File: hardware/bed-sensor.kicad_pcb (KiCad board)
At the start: 2 copper layers, 21.3 x 43.2 mm, 46 parts, among them J1 USB_B_Mini, J2 Conn_ARM_JTAG_SWD_10, J3 DM3AT-SF-PEJM5, J4 Conn_01x02, Q1 Q_PMOS_GSD, SW1 SW_Push, U1 MCP73831-2-OT, U2 TLV70218_SOT23-5, U3 AP2112K-3.3, U4 MDBT50Q-1M, U5 PCA9306, U6 ICM-20948, U7 BMP280, Y1 32.768

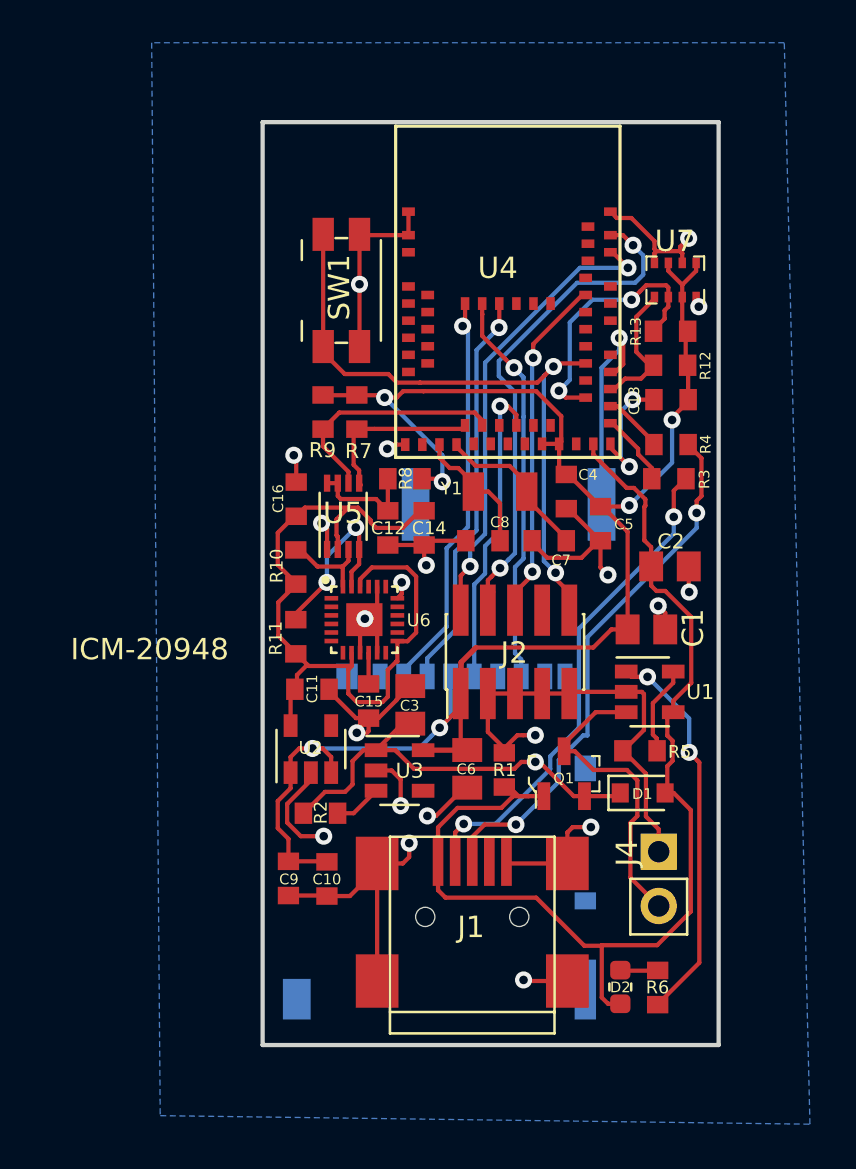
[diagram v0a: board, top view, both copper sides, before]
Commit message: finalized order list
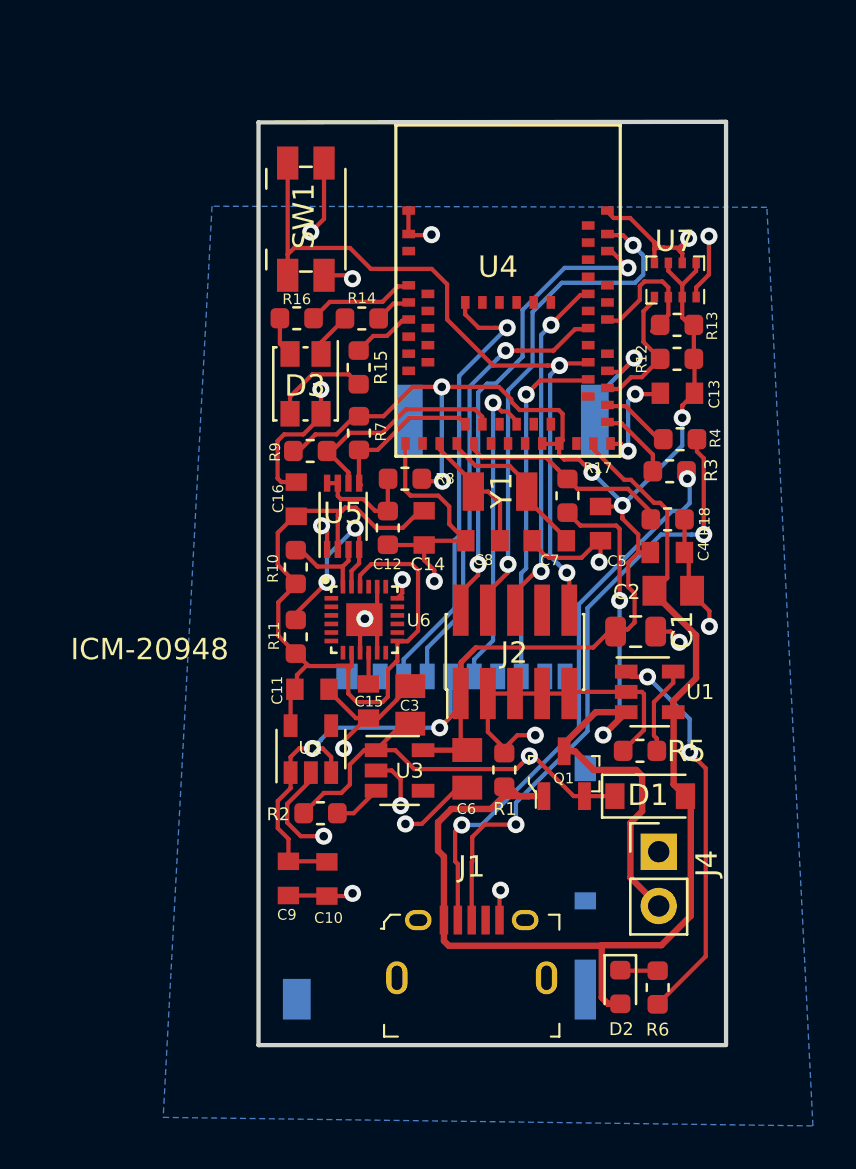
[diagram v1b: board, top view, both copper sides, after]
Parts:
- added D3: LED_RCGB, LED_SMD:LED_Kingbright_AAA3528ESGCT, F.Cu at (138.6, 98.6)
- added R14: 330, Resistor_SMD:R_0603_1608Metric, F.Cu at (141.2, 95.5)
- added R15: 330, Resistor_SMD:R_0603_1608Metric, F.Cu at (141.1, 97.8)
- added R16: 330, Resistor_SMD:R_0603_1608Metric, F.Cu at (138.2, 95.5)
- added R17: 100k, Resistor_SMD:R_0603_1608Metric, F.Cu at (150.8, 103.8)
- added R18: 100k, Resistor_SMD:R_0603_1608Metric, F.Cu at (155.5, 105.0)
- D1: footprint Diodes_SMD:D_0805 -> Diode_SMD:D_SOD-123
- D2: footprint Capacitor_SMD:C_0603_1608Metric -> Diode_SMD:D_0603_1608Metric
- J1: footprint Connectors:USB_Mini-B -> digikey-footprints:USB_Micro_B_Female_10118194-0001LF
- moved C4 5.52 mm to (155.5, 106.5), turned to 0 degrees
- moved BZ1 3.91 mm to (147.8, 100.3)
- moved SW1 3.73 mm to (138.6, 90.9)
- moved R9 1.92 mm to (138.8, 101.8), turned to 180 degrees
- moved C2 1.15 mm to (155.8, 108.3)
- moved R7 0.99 mm to (141.1, 100.9)
- moved C1 0.51 mm to (154.0, 110.2)
- moved R4 0.49 mm to (156.1, 101.2)
- moved R13 0.42 mm to (156.0, 95.8)
- moved R12 0.42 mm to (156.0, 97.4)
- moved C13 0.42 mm to (156.0, 99.0)
- moved D1 0.38 mm to (154.7, 117.9)
- moved R3 0.35 mm to (155.6, 102.7)
- moved J1 0.06 mm to (146.3, 123.7), turned to 0 degrees
- moved U4 0.05 mm to (142.8, 102.0)
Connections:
- J1 pad 4: Net-(J1-Pad4) -> (no net)
- J2 pad 8: Net-(J2-Pad8) -> (no net)
- J3 pad 1: Net-(J3-Pad1) -> (no net)
- J3 pad 8: Net-(J3-Pad8) -> (no net)
- J3 pad SWA: Net-(J3-PadSWA) -> (no net)
- J3 pad SWB: Net-(J3-PadSWB) -> (no net)
- U2 pad 4: Net-(U2-Pad4) -> (no net)
- U3 pad 4: Net-(U3-Pad4) -> (no net)
- U4 pad 10: Net-(U4-Pad10) -> (no net)
- U4 pad 11: Net-(U4-Pad11) -> (no net)
- U4 pad 12: Net-(U4-Pad12) -> (no net)
- U4 pad 13: Net-(U4-Pad13) -> (no net)
- U4 pad 14: Net-(U4-Pad14) -> (no net)
- U4 pad 16: Net-(U4-Pad16) -> (no net)
- U4 pad 20: Net-(U4-Pad20) -> VDIV
- U4 pad 22: Net-(U4-Pad22) -> (no net)
- U4 pad 23: Net-(U4-Pad23) -> (no net)
- U4 pad 24: Net-(U4-Pad24) -> (no net)
- U4 pad 26: Net-(U4-Pad26) -> (no net)
- U4 pad 27: Net-(U4-Pad27) -> (no net)
- U4 pad 29: Net-(U4-Pad29) -> (no net)
- U4 pad 3: Net-(U4-Pad3) -> (no net)
- U4 pad 31: Net-(U4-Pad31) -> (no net)
- U4 pad 36: BMP_SDA -> (no net)
- U4 pad 38: Net-(U4-Pad38) -> SD_MISO
- U4 pad 4: Net-(U4-Pad4) -> B_LED
- U4 pad 41: Net-(U4-Pad41) -> (no net)
- U4 pad 42: Net-(U4-Pad42) -> (no net)
- U4 pad 43: Net-(U4-Pad43) -> SD_MOSI
- U4 pad 44: Net-(U4-Pad44) -> BMP_SDA
- U4 pad 45: Net-(U4-Pad45) -> (no net)
- U4 pad 46: Net-(U4-Pad46) -> (no net)
- U4 pad 48: Net-(U4-Pad48) -> (no net)
- U4 pad 5: Net-(U4-Pad5) -> (no net)
- U4 pad 50: Net-(U4-Pad50) -> (no net)
- U4 pad 52: Net-(U4-Pad52) -> (no net)
- U4 pad 54: Net-(U4-Pad54) -> (no net)
- U4 pad 57: SD_MISO -> (no net)
- U4 pad 58: SD_MOSI -> (no net)
- U4 pad 59: Net-(U4-Pad59) -> (no net)
- U4 pad 6: Net-(U4-Pad6) -> R_LED
- U4 pad 60: Net-(U4-Pad60) -> (no net)
- U4 pad 61: Net-(U4-Pad61) -> (no net)
- U4 pad 7: Net-(U4-Pad7) -> (no net)
- U4 pad 8: Net-(U4-Pad8) -> G_LED
- U4 pad 9: Net-(U4-Pad9) -> (no net)
- U6 pad 12: Net-(U6-Pad12) -> (no net)
- U6 pad 19: Net-(U6-Pad19) -> (no net)
- U6 pad 21: Net-(U6-Pad21) -> (no net)
- U6 pad 7: Net-(U6-Pad7) -> (no net)
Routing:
- net +BATT: track 14.6 -> 29.4 mm, vias 0 -> 2
- net VDIV: track 0.00 -> 10.3 mm
- net BMP_SDA: track 12.9 -> 6.33 mm, vias 2 -> 0
- net GND: track 105.9 -> 100.3 mm
- net BUZZER: track 10.2 -> 5.12 mm
- net B_LED: track 0.00 -> 5.06 mm
- net +3V3: track 83.0 -> 87.7 mm, vias 6 -> 7
- net Net-(D3-Pad3): track 0.00 -> 4.63 mm
- net USB_D+: track 25.2 -> 29.2 mm
- net RESET: track 31.1 -> 34.8 mm
- net USB_D-: track 23.2 -> 26.2 mm
- net G_LED: track 0.00 -> 2.91 mm
- net SD_CS: track 18.8 -> 21.1 mm
- net SD_MISO: track 18.5 -> 16.3 mm
- net VBUS: track 51.9 -> 54.1 mm
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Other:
- board size 21.3 x 43.2 mm -> 21.9 x 43.2 mm
